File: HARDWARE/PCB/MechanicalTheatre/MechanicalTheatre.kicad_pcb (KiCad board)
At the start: 2 copper layers, 4 parts, among them U1 Teensy4.1, U2 SN74AHCT125N, U3 ESP32-DEVKITC-32D, U4 SN74HC14N

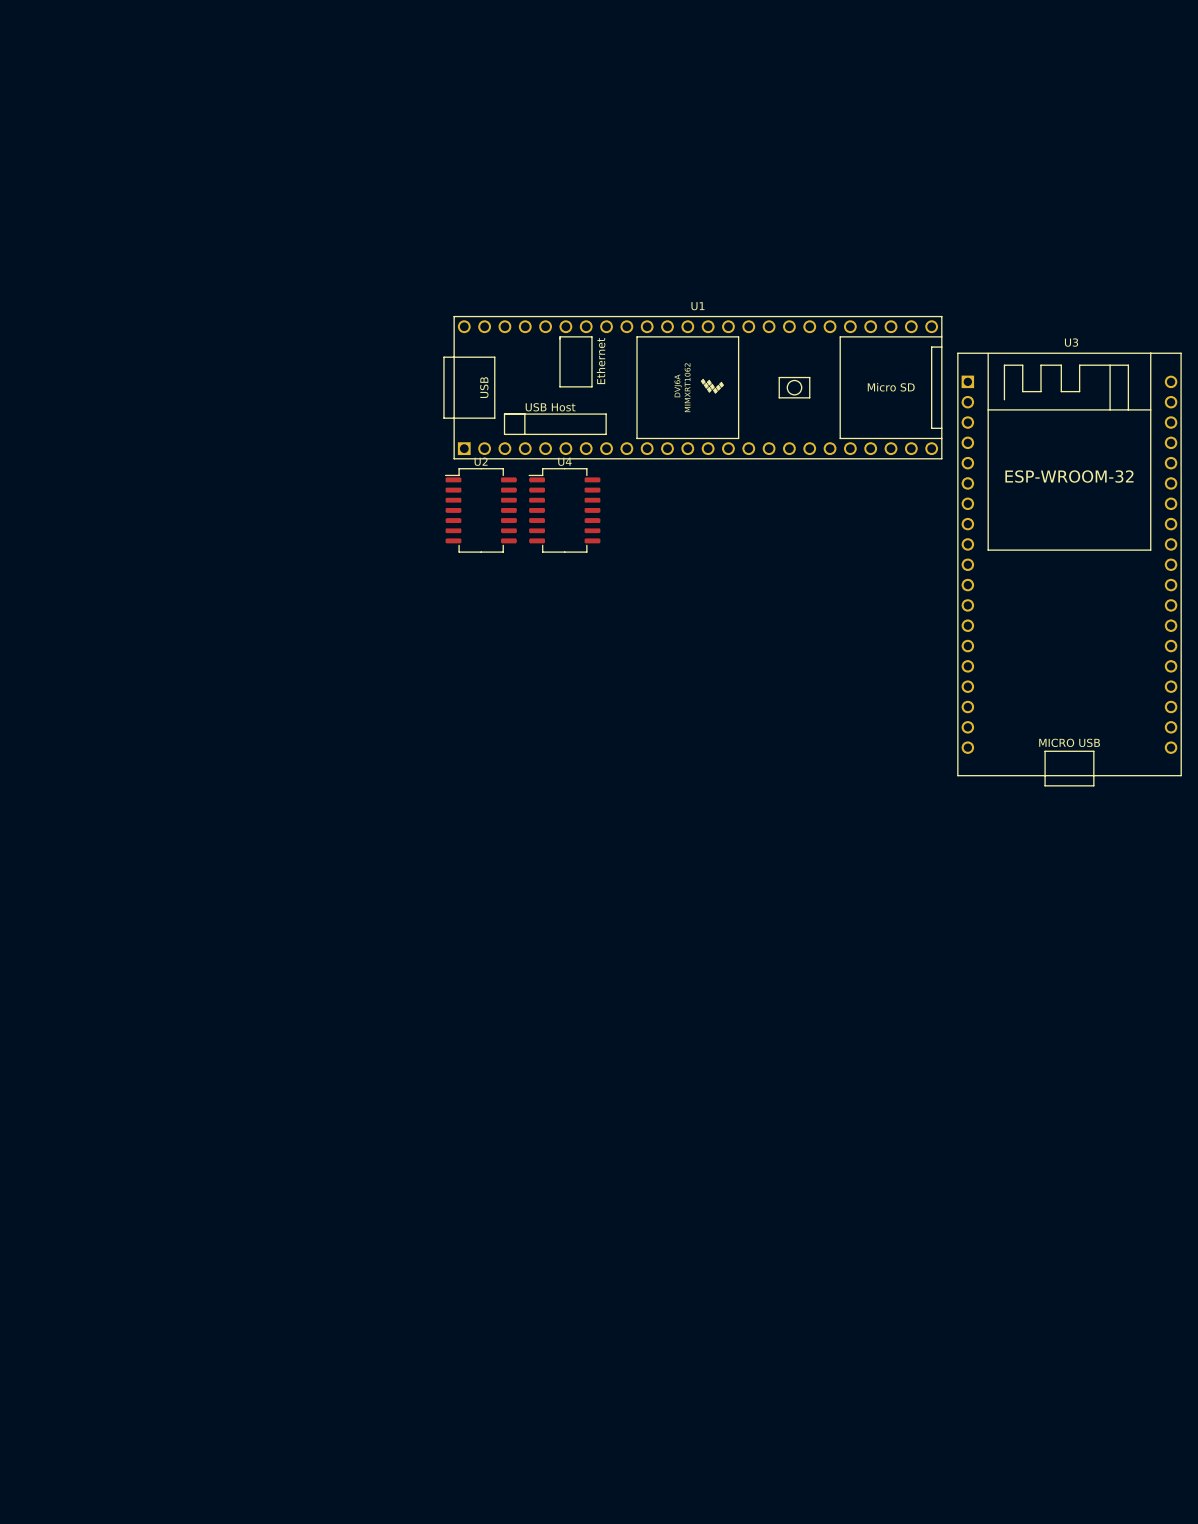
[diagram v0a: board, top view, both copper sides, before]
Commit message: main pcb v1.0
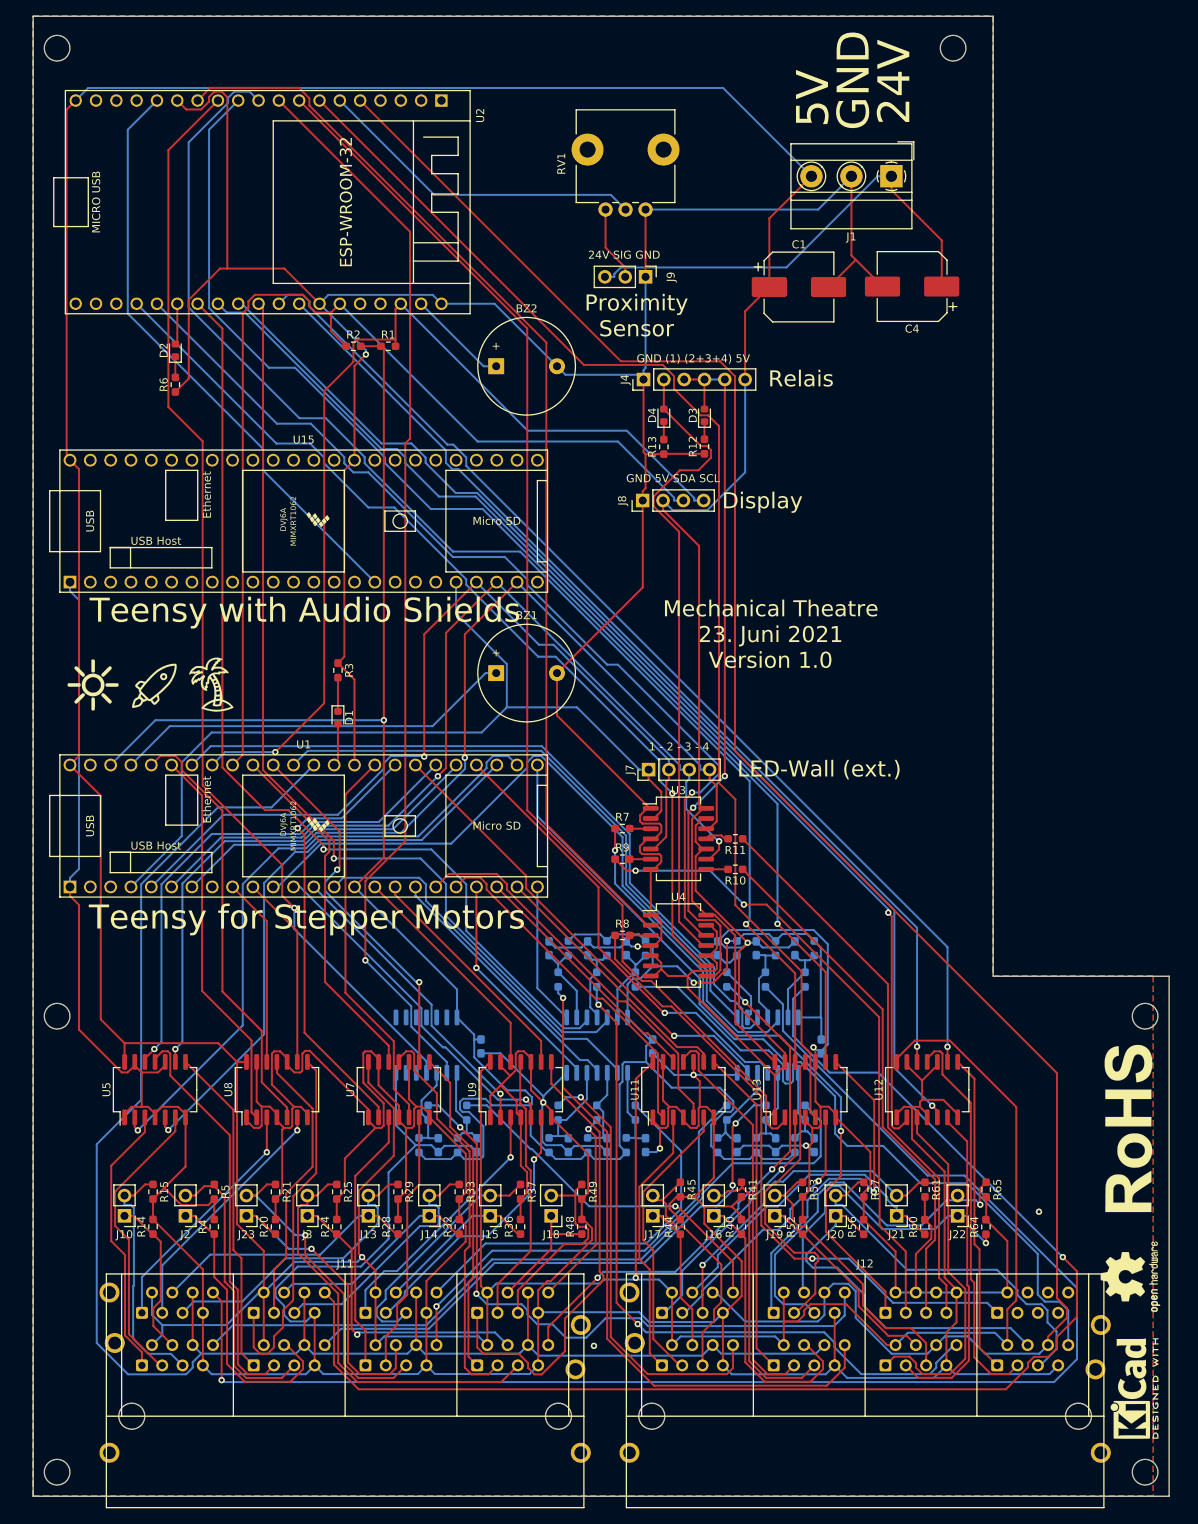
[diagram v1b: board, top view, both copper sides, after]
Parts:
- added BZ1: Buzzer, Buzzer_Beeper:Buzzer_12x9.5RM7.6, F.Cu at (87.9, 122.1)
- added BZ2: Buzzer, Buzzer_Beeper:Buzzer_12x9.5RM7.6, F.Cu at (87.9, 83.8)
- added C1: 220uF, 25V, Capacitor_SMD:CP_Elec_8x10.5, F.Cu at (125.7, 73.9)
- added C10: 0.1uF 16V, Capacitor_SMD:C_0603_1608Metric_Pad1.08x0.95mm_HandSolder, B.Cu at (107.4, 168.8)
- added C11: 0.1uF 16V, Capacitor_SMD:C_0603_1608Metric_Pad1.08x0.95mm_HandSolder, B.Cu at (106.6, 181.1)
- added C12: 0.1uF 16V, Capacitor_SMD:C_0603_1608Metric_Pad1.08x0.95mm_HandSolder, B.Cu at (94.5, 156.5)
- added C13: 0.1uF 16V, Capacitor_SMD:C_0603_1608Metric_Pad1.08x0.95mm_HandSolder, B.Cu at (96.9, 181.1)
- added C14: 0.1uF 16V, Capacitor_SMD:C_0603_1608Metric_Pad1.08x0.95mm_HandSolder, B.Cu at (101.7, 181.1)
- added C15: 0.1uF 16V, Capacitor_SMD:C_0603_1608Metric_Pad1.08x0.95mm_HandSolder, B.Cu at (99.3, 156.5)
- added C16: 0.1uF 16V, Capacitor_SMD:C_0603_1608Metric_Pad1.08x0.95mm_HandSolder, B.Cu at (104.1, 156.5)
- added C17: 0.1uF 16V, Capacitor_SMD:C_0603_1608Metric_Pad1.08x0.95mm_HandSolder, B.Cu at (86.0, 168.8)
- added C18: 0.1uF 16V, Capacitor_SMD:C_0603_1608Metric_Pad1.08x0.95mm_HandSolder, B.Cu at (85.5, 181.1)
- added C2: 0.1uF 16V, Capacitor_SMD:C_0603_1608Metric_Pad1.08x0.95mm_HandSolder, B.Cu at (122.8, 181.1)
- added C20: 0.1uF 16V, Capacitor_SMD:C_0603_1608Metric_Pad1.08x0.95mm_HandSolder, B.Cu at (80.6, 181.1)
- added C3: 0.1uF 16V, Capacitor_SMD:C_0603_1608Metric_Pad1.08x0.95mm_HandSolder, B.Cu at (118.0, 181.1)
- added C4: 220uF, 25V, Capacitor_SMD:CP_Elec_8x10.5, F.Cu at (139.9, 73.8)
- added C5: 0.1uF 16V, Capacitor_SMD:C_0603_1608Metric_Pad1.08x0.95mm_HandSolder, B.Cu at (128.5, 168.8)
- added C6: 0.1uF 16V, Capacitor_SMD:C_0603_1608Metric_Pad1.08x0.95mm_HandSolder, B.Cu at (127.6, 181.1)
- added C7: 0.1uF 16V, Capacitor_SMD:C_0603_1608Metric_Pad1.08x0.95mm_HandSolder, B.Cu at (115.6, 156.5)
- added C8: 0.1uF 16V, Capacitor_SMD:C_0603_1608Metric_Pad1.08x0.95mm_HandSolder, B.Cu at (120.4, 156.5)
- added C9: 0.1uF 16V, Capacitor_SMD:C_0603_1608Metric_Pad1.08x0.95mm_HandSolder, B.Cu at (125.2, 156.5)
- added D1: LED, LED_SMD:LED_0603_1608Metric, F.Cu at (68.1, 127.7)
- added D2: LED, LED_SMD:LED_0603_1608Metric, F.Cu at (47.8, 81.8)
- added D3: LED, LED_SMD:LED_0603_1608Metric, F.Cu at (113.9, 89.9)
- added D4: LED, LED_SMD:LED_0603_1608Metric, F.Cu at (108.8, 89.9)
- added G***: LOGO, Clockdiv-Logos:sunrocketpalmtree_21.7mm, F.Cu at (44.7, 123.9)
- added J1: Power In 5V/24V, TerminalBlock_MetzConnect:TerminalBlock_MetzConnect_Type011_RT05503HBWC_1x03_P5.00mm_Horizontal, F.Cu at (137.3, 60.0)
- added J10: Conn_01x02_General Purpose 01, Connector_PinHeader_2.54mm:PinHeader_1x02_P2.54mm_Vertical, F.Cu at (41.4, 190.0)
- added J11: RJ45 8x Socket, Clockdiv-KiCad:RJ45_Conrad_8x, F.Cu at (69.0, 215.0)
- added J12: RJ45 8x Socket, Clockdiv-KiCad:RJ45_Conrad_8x, F.Cu at (134.0, 215.0)
- added J13: Conn_01x02_General Purpose 05, Connector_PinHeader_2.54mm:PinHeader_1x02_P2.54mm_Vertical, F.Cu at (71.9, 190.0)
- added J14: Conn_01x02_General Purpose 06, Connector_PinHeader_2.54mm:PinHeader_1x02_P2.54mm_Vertical, F.Cu at (79.5, 190.0)
- added J15: Conn_01x02_General Purpose 07, Connector_PinHeader_2.54mm:PinHeader_1x02_P2.54mm_Vertical, F.Cu at (87.1, 190.0)
- added J16: Conn_01x02_General Purpose 10, Connector_PinHeader_2.54mm:PinHeader_1x02_P2.54mm_Vertical, F.Cu at (115.1, 190.0)
- added J17: Conn_01x02_General Purpose 09, Connector_PinHeader_2.54mm:PinHeader_1x02_P2.54mm_Vertical, F.Cu at (107.5, 190.0)
- added J18: Conn_01x02_General Purpose 08, Connector_PinHeader_2.54mm:PinHeader_1x02_P2.54mm_Vertical, F.Cu at (94.8, 190.0)
- added J19: Conn_01x02_General Purpose 11, Connector_PinHeader_2.54mm:PinHeader_1x02_P2.54mm_Vertical, F.Cu at (122.7, 190.0)
- added J2: Conn_01x02_General Purpose 02, Connector_PinHeader_2.54mm:PinHeader_1x02_P2.54mm_Vertical, F.Cu at (49.0, 190.0)
- added J20: Conn_01x02_General Purpose 12, Connector_PinHeader_2.54mm:PinHeader_1x02_P2.54mm_Vertical, F.Cu at (130.3, 190.0)
- added J21: Conn_01x02_General Purpose 13, Connector_PinHeader_2.54mm:PinHeader_1x02_P2.54mm_Vertical, F.Cu at (137.9, 190.0)
- added J22: Conn_01x02_General Purpose 14, Connector_PinHeader_2.54mm:PinHeader_1x02_P2.54mm_Vertical, F.Cu at (145.6, 190.0)
- added J23: Conn_01x02_General Purpose 03, Connector_PinHeader_2.54mm:PinHeader_1x02_P2.54mm_Vertical, F.Cu at (56.7, 190.0)
- added J3: Conn_01x02_General Purpose 04, Connector_PinHeader_2.54mm:PinHeader_1x02_P2.54mm_Vertical, F.Cu at (64.3, 190.0)
- added J4: Conn_01x06_Relais, Connector_PinHeader_2.54mm:PinHeader_1x06_P2.54mm_Vertical, F.Cu at (106.3, 85.4)
- added J7: Conn_01x04_WS2812B, Connector_PinHeader_2.54mm:PinHeader_1x04_P2.54mm_Vertical, F.Cu at (106.9, 134.2)
- added J8: Conn_01x04_I2C_Display_20x4, Connector_PinHeader_2.54mm:PinHeader_1x04_P2.54mm_Vertical, F.Cu at (106.2, 100.5)
- added J9: Conn_01x03_ProximitySensor, Connector_PinHeader_2.54mm:PinHeader_1x03_P2.54mm_Vertical, F.Cu at (106.6, 72.6)
- added R1: 4.7k, Resistor_SMD:R_0603_1608Metric_Pad0.98x0.95mm_HandSolder, F.Cu at (74.4, 81.3)
- added R10: 100, Resistor_SMD:R_0603_1608Metric_Pad0.98x0.95mm_HandSolder, F.Cu at (117.8, 146.6)
- added R11: 100, Resistor_SMD:R_0603_1608Metric_Pad0.98x0.95mm_HandSolder, F.Cu at (117.8, 142.8)
- added R12: 120, Resistor_SMD:R_0603_1608Metric_Pad0.98x0.95mm_HandSolder, F.Cu at (113.9, 93.8)
- added R13: 120, Resistor_SMD:R_0603_1608Metric_Pad0.98x0.95mm_HandSolder, F.Cu at (108.8, 93.8)
- added R14: 10k, Resistor_SMD:R_0603_1608Metric_Pad0.98x0.95mm_HandSolder, F.Cu at (45.0, 191.3)
- added R15: 10k, Resistor_SMD:R_0603_1608Metric_Pad0.98x0.95mm_HandSolder, F.Cu at (45.0, 186.9)
- added R16: 10k, Resistor_SMD:R_0603_1608Metric_Pad0.98x0.95mm_HandSolder, B.Cu at (125.2, 181.1)
- added R17: 1k, Resistor_SMD:R_0603_1608Metric_Pad0.98x0.95mm_HandSolder, B.Cu at (126.5, 177.1)
- added R18: 10k, Resistor_SMD:R_0603_1608Metric_Pad0.98x0.95mm_HandSolder, B.Cu at (120.4, 181.1)
- added R19: 1k, Resistor_SMD:R_0603_1608Metric_Pad0.98x0.95mm_HandSolder, B.Cu at (121.6, 177.1)
- added R2: 4.7k, Resistor_SMD:R_0603_1608Metric_Pad0.98x0.95mm_HandSolder, F.Cu at (70.0, 81.3)
- added R20: 10k, Resistor_SMD:R_0603_1608Metric_Pad0.98x0.95mm_HandSolder, F.Cu at (60.3, 191.3)
- added R21: 10k, Resistor_SMD:R_0603_1608Metric_Pad0.98x0.95mm_HandSolder, F.Cu at (60.3, 186.9)
- added R22: 10k, Resistor_SMD:R_0603_1608Metric_Pad0.98x0.95mm_HandSolder, B.Cu at (115.6, 181.1)
- added R23: 1k, Resistor_SMD:R_0603_1608Metric_Pad0.98x0.95mm_HandSolder, B.Cu at (116.7, 177.1)
- added R24: 10k, Resistor_SMD:R_0603_1608Metric_Pad0.98x0.95mm_HandSolder, F.Cu at (68.0, 191.3)
- added R25: 10k, Resistor_SMD:R_0603_1608Metric_Pad0.98x0.95mm_HandSolder, F.Cu at (68.0, 186.9)
- added R26: 10k, Resistor_SMD:R_0603_1608Metric_Pad0.98x0.95mm_HandSolder, B.Cu at (118.0, 156.5)
- added R27: 1k, Resistor_SMD:R_0603_1608Metric_Pad0.98x0.95mm_HandSolder, B.Cu at (116.7, 160.4)
- added R28: 10k, Resistor_SMD:R_0603_1608Metric_Pad0.98x0.95mm_HandSolder, F.Cu at (75.6, 191.3)
- added R29: 10k, Resistor_SMD:R_0603_1608Metric_Pad0.98x0.95mm_HandSolder, F.Cu at (75.6, 186.9)
- added R3: 220, Resistor_SMD:R_0603_1608Metric_Pad0.98x0.95mm_HandSolder, F.Cu at (68.1, 121.8)
- added R30: 10k, Resistor_SMD:R_0603_1608Metric_Pad0.98x0.95mm_HandSolder, B.Cu at (122.8, 156.5)
- added R31: 1k, Resistor_SMD:R_0603_1608Metric_Pad0.98x0.95mm_HandSolder, B.Cu at (121.5, 160.4)
- added R32: 10k, Resistor_SMD:R_0603_1608Metric_Pad0.98x0.95mm_HandSolder, F.Cu at (83.3, 191.3)
- added R33: 10k, Resistor_SMD:R_0603_1608Metric_Pad0.98x0.95mm_HandSolder, F.Cu at (83.3, 186.9)
- added R34: 10k, Resistor_SMD:R_0603_1608Metric_Pad0.98x0.95mm_HandSolder, B.Cu at (127.6, 156.5)
- added R35: 1k, Resistor_SMD:R_0603_1608Metric_Pad0.98x0.95mm_HandSolder, B.Cu at (126.5, 160.4)
- added R36: 10k, Resistor_SMD:R_0603_1608Metric_Pad0.98x0.95mm_HandSolder, F.Cu at (90.9, 191.3)
- added R37: 10k, Resistor_SMD:R_0603_1608Metric_Pad0.98x0.95mm_HandSolder, F.Cu at (90.9, 186.9)
- added R38: 10k, Resistor_SMD:R_0603_1608Metric_Pad0.98x0.95mm_HandSolder, B.Cu at (104.1, 181.1)
- added R39: 1k, Resistor_SMD:R_0603_1608Metric_Pad0.98x0.95mm_HandSolder, B.Cu at (105.3, 177.1)
- added R4: 10k, Resistor_SMD:R_0603_1608Metric_Pad0.98x0.95mm_HandSolder, F.Cu at (52.6, 191.3)
- added R40: 10k, Resistor_SMD:R_0603_1608Metric_Pad0.98x0.95mm_HandSolder, F.Cu at (118.5, 191.3)
- added R41: 10k, Resistor_SMD:R_0603_1608Metric_Pad0.98x0.95mm_HandSolder, F.Cu at (118.5, 186.7)
- added R42: 10k, Resistor_SMD:R_0603_1608Metric_Pad0.98x0.95mm_HandSolder, B.Cu at (96.9, 156.5)
- added R43: 1k, Resistor_SMD:R_0603_1608Metric_Pad0.98x0.95mm_HandSolder, B.Cu at (95.6, 160.4)
- added R44: 10k, Resistor_SMD:R_0603_1608Metric_Pad0.98x0.95mm_HandSolder, F.Cu at (110.9, 191.3)
- added R45: 10k, Resistor_SMD:R_0603_1608Metric_Pad0.98x0.95mm_HandSolder, F.Cu at (110.9, 186.7)
- added R46: 10k, Resistor_SMD:R_0603_1608Metric_Pad0.98x0.95mm_HandSolder, B.Cu at (94.5, 181.1)
- added R47: 1k, Resistor_SMD:R_0603_1608Metric_Pad0.98x0.95mm_HandSolder, B.Cu at (95.6, 177.1)
- added R48: 10k, Resistor_SMD:R_0603_1608Metric_Pad0.98x0.95mm_HandSolder, F.Cu at (98.6, 191.3)
- added R49: 10k, Resistor_SMD:R_0603_1608Metric_Pad0.98x0.95mm_HandSolder, F.Cu at (98.6, 186.9)
- added R5: 10k, Resistor_SMD:R_0603_1608Metric_Pad0.98x0.95mm_HandSolder, F.Cu at (52.6, 186.9)
- added R50: 10k, Resistor_SMD:R_0603_1608Metric_Pad0.98x0.95mm_HandSolder, B.Cu at (99.3, 181.1)
- added R51: 1k, Resistor_SMD:R_0603_1608Metric_Pad0.98x0.95mm_HandSolder, B.Cu at (100.5, 177.1)
- added R52: 10k, Resistor_SMD:R_0603_1608Metric_Pad0.98x0.95mm_HandSolder, F.Cu at (126.2, 191.3)
- added R53: 10k, Resistor_SMD:R_0603_1608Metric_Pad0.98x0.95mm_HandSolder, F.Cu at (126.2, 186.7)
- added R54: 10k, Resistor_SMD:R_0603_1608Metric_Pad0.98x0.95mm_HandSolder, B.Cu at (101.7, 156.5)
- added R55: 1k, Resistor_SMD:R_0603_1608Metric_Pad0.98x0.95mm_HandSolder, B.Cu at (100.5, 160.4)
- added R56: 10k, Resistor_SMD:R_0603_1608Metric_Pad0.98x0.95mm_HandSolder, F.Cu at (133.8, 191.3)
- added R57: 10k, Resistor_SMD:R_0603_1608Metric_Pad0.98x0.95mm_HandSolder, F.Cu at (133.8, 186.7)
- added R58: 10k, Resistor_SMD:R_0603_1608Metric_Pad0.98x0.95mm_HandSolder, B.Cu at (106.6, 156.5)
- added R59: 1k, Resistor_SMD:R_0603_1608Metric_Pad0.98x0.95mm_HandSolder, B.Cu at (105.3, 160.4)
- added R6: 120, Resistor_SMD:R_0603_1608Metric_Pad0.98x0.95mm_HandSolder, F.Cu at (47.8, 86.1)
- added R60: 10k, Resistor_SMD:R_0603_1608Metric_Pad0.98x0.95mm_HandSolder, F.Cu at (141.5, 191.3)
- added R61: 10k, Resistor_SMD:R_0603_1608Metric_Pad0.98x0.95mm_HandSolder, F.Cu at (141.5, 186.7)
- added R62: 10k, Resistor_SMD:R_0603_1608Metric_Pad0.98x0.95mm_HandSolder, B.Cu at (83.1, 181.1)
- added R63: 1k, Resistor_SMD:R_0603_1608Metric_Pad0.98x0.95mm_HandSolder, B.Cu at (84.2, 177.1)
- added R64: 10k, Resistor_SMD:R_0603_1608Metric_Pad0.98x0.95mm_HandSolder, F.Cu at (149.1, 191.3)
- added R65: 10k, Resistor_SMD:R_0603_1608Metric_Pad0.98x0.95mm_HandSolder, F.Cu at (149.1, 186.7)
- added R66: 10k, Resistor_SMD:R_0603_1608Metric_Pad0.98x0.95mm_HandSolder, B.Cu at (78.2, 181.1)
- added R67: 1k, Resistor_SMD:R_0603_1608Metric_Pad0.98x0.95mm_HandSolder, B.Cu at (79.4, 177.1)
- added R7: 100, Resistor_SMD:R_0603_1608Metric_Pad0.98x0.95mm_HandSolder, F.Cu at (103.7, 141.5)
- added R8: 100, Resistor_SMD:R_0603_1608Metric_Pad0.98x0.95mm_HandSolder, F.Cu at (103.7, 154.9)
- added R9: 100, Resistor_SMD:R_0603_1608Metric_Pad0.98x0.95mm_HandSolder, F.Cu at (103.7, 145.4)
- added REF**: OSHW-Logo2_9.8x8mm_SilkScreen, Symbol:OSHW-Logo2_9.8x8mm_SilkScreen, F.Cu at (167.2, 197.6)
- added REF**: KiCad-Logo2_5mm_SilkScreen, Symbol:KiCad-Logo2_5mm_SilkScreen, F.Cu at (167.7, 211.5)
- added REF**: RoHS-Logo_6mm_SilkScreen, Symbol:RoHS-Logo_6mm_SilkScreen, F.Cu at (166.9, 179.0)
- added RV1: R_POT, Potentiometer_THT:Potentiometer_Alps_RK09L_Single_Vertical, F.Cu at (106.6, 64.2)
- added U10: SN74HC14S, Package_SO:SO-14_5.3x10.2mm_P1.27mm, B.Cu at (100.5, 168.6)
- added U11: SN74AHCT125N, Package_SO:SO-14_5.3x10.2mm_P1.27mm, F.Cu at (111.3, 174.2)
- added U12: SN74AHCT125N, Package_SO:SO-14_5.3x10.2mm_P1.27mm, F.Cu at (141.8, 174.2)
- added U13: SN74AHCT125N, Package_SO:SO-14_5.3x10.2mm_P1.27mm, F.Cu at (126.5, 174.2)
- added U14: SN74HC14S, Package_SO:SO-14_5.3x10.2mm_P1.27mm, B.Cu at (79.2, 168.6)
- added U15: Teensy4.1_OuterPins, teensy:Teensy41_OuterPinsOnly, F.Cu at (63.8, 103.1)
- added U5: SN74AHCT125N, Package_SO:SO-14_5.3x10.2mm_P1.27mm, F.Cu at (45.2, 174.2)
- added U6: SN74HC14S, Package_SO:SO-14_5.3x10.2mm_P1.27mm, B.Cu at (121.8, 168.6)
- added U7: SN74AHCT125N, Package_SO:SO-14_5.3x10.2mm_P1.27mm, F.Cu at (75.7, 174.2)
- added U8: SN74AHCT125N, Package_SO:SO-14_5.3x10.2mm_P1.27mm, F.Cu at (60.5, 174.2)
- added U9: SN74AHCT125N, Package_SO:SO-14_5.3x10.2mm_P1.27mm, F.Cu at (91.0, 174.2)
- U1: value Teensy4.1 -> Teensy4.1_OuterPins
- U2: value SN74AHCT125N -> ESP32-DEVKITC-32D; footprint Package_SO:SO-14_5.3x10.2mm_P1.27mm -> ESP32-DEVKITC-32D:MODULE_ESP32-DEVKITC-32D
- U3: value ESP32-DEVKITC-32D -> SN74AHCT125N; footprint ESP32-DEVKITC-32D:MODULE_ESP32-DEVKITC-32D -> Package_SO:SO-14_5.3x10.2mm_P1.27mm
- U4: value SN74HC14N -> SN74AHCT125N
- moved U1 73.7 mm to (63.8, 141.2)
- moved U3 61.5 mm to (110.7, 142.8)
- moved U4 56.2 mm to (110.7, 156.2)
- moved U2 45.8 mm to (61.3, 63.2), turned to 270 degrees
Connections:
- U1 pad 1: Net-(U1-Pad1) -> GND
- U1 pad 10: Net-(U1-Pad10) -> /STEPPER_6_DIR
- U1 pad 11: Net-(U1-Pad11) -> /STEPPER_6_END
- U1 pad 12: Net-(U1-Pad12) -> /STEPPER_7_STEP
- U1 pad 13: Net-(U1-Pad13) -> /STEPPER_7_DIR
- U1 pad 14: Net-(U1-Pad14) -> /STEPPER_7_END
- U1 pad 15: Net-(U1-Pad15) -> +3V3
- U1 pad 16: Net-(U1-Pad16) -> /STEPPER_8_STEP
- U1 pad 17: Net-(U1-Pad17) -> /STEPPER_8_DIR
- U1 pad 18: Net-(U1-Pad18) -> /STEPPER_8_END
- U1 pad 19: Net-(U1-Pad19) -> /STEPPER_9_STEP
- U1 pad 20: Net-(U1-Pad20) -> /STEPPER_9_DIR
- U1 pad 21: Net-(U1-Pad21) -> /STEPPER_9_END
- U1 pad 22: Net-(U1-Pad22) -> /STEPPER_10_STEP
- U1 pad 23: Net-(U1-Pad23) -> /STEPPER_10_DIR
- U1 pad 24: Net-(U1-Pad24) -> /STEPPER_10_END
- U1 pad 25: Net-(U1-Pad25) -> /STEPPER_1_END
- U1 pad 26: Net-(U1-Pad26) -> /STEPPER_1_DIR
- U1 pad 27: Net-(U1-Pad27) -> /STEPPER_1_STEP
- U1 pad 28: Net-(U1-Pad28) -> /STEPPER_2_END
- U1 pad 29: Net-(U1-Pad29) -> /STEPPER_2_DIR
- U1 pad 30: Net-(U1-Pad30) -> /STEPPER_2_STEP
- U1 pad 31: Net-(U1-Pad31) -> /STEPPER_3_END
- U1 pad 32: Net-(U1-Pad32) -> /STEPPER_3_DIR
- U1 pad 33: Net-(U1-Pad33) -> /STEPPER_3_STEP
- U1 pad 34: Net-(U1-Pad34) -> GND
- U1 pad 36: Net-(U1-Pad36) -> /GENERAL_END_SWITCH_TEENSY
- U1 pad 37: Net-(U1-Pad37) -> /STEPPER_4_END
- U1 pad 38: Net-(U1-Pad38) -> /STEPPER_4_DIR
- U1 pad 39: Net-(U1-Pad39) -> /STEPPER_4_STEP
- U1 pad 4: Net-(U1-Pad4) -> /WS2812B_Line_1
- U1 pad 40: Net-(U1-Pad40) -> /I2C_SDA
- U1 pad 41: Net-(U1-Pad41) -> /I2C_SCL
- U1 pad 42: Net-(U1-Pad42) -> /STEPPER_5_END
- U1 pad 43: Net-(U1-Pad43) -> /STEPPER_5_DIR
- U1 pad 44: Net-(U1-Pad44) -> /STEPPER_5_STEP
- U1 pad 46: Net-(U1-Pad46) -> +3V3
- U1 pad 48: Net-(U1-Pad48) -> +5V
- U1 pad 5: Net-(U1-Pad5) -> /WS2812B_Line_2
- U1 pad 6: Net-(U1-Pad6) -> /WS2812B_Line_3
- U1 pad 7: Net-(U1-Pad7) -> /WS2812B_Line_4
- U1 pad 9: Net-(U1-Pad9) -> /STEPPER_6_STEP
- U2 pad 10: Net-(U2-Pad10) -> /STEPPER_14_STEP
- U2 pad 11: Net-(U2-Pad11) -> /STEPPER_14_DIR
- U2 pad 12: Net-(U2-Pad12) -> /STEPPER_14_END
- U2 pad 13: Net-(U2-Pad13) -> /WS2812B_LED_LIGHTING
- U2 pad 14: Net-(U2-Pad14) -> GND
- U2 pad 5: Net-(U2-Pad5) -> /GENERAL_END_SWITCH_ESP32
- U2 pad 6: Net-(U2-Pad6) -> /PROX_SENSOR
- U2 pad 7: Net-(U2-Pad7) -> /STEPPER_13_STEP
- U2 pad 8: Net-(U2-Pad8) -> /STEPPER_13_DIR
- U2 pad 9: Net-(U2-Pad9) -> /STEPPER_13_END
- U3 pad 1: Net-(U3-Pad1) -> GND
- U3 pad 10: Net-(U3-Pad10) -> GND
- U3 pad 12: Net-(U3-Pad12) -> /WS2812B_Line_4
- U3 pad 13: Net-(U3-Pad13) -> GND
- U3 pad 14: Net-(U3-Pad14) -> +5V
- U3 pad 2: Net-(U3-Pad2) -> /WS2812B_Line_1
- U3 pad 4: Net-(U3-Pad4) -> GND
- U3 pad 5: Net-(U3-Pad5) -> /WS2812B_Line_2
- U3 pad 7: Net-(U3-Pad7) -> GND
- U3 pad 9: Net-(U3-Pad9) -> /WS2812B_Line_3
- U4 pad 1: Net-(U4-Pad1) -> GND
- U4 pad 10: Net-(U4-Pad10) -> GND
- U4 pad 12: Net-(U4-Pad12) -> /RELAIS_E-MAGNET
- U4 pad 13: Net-(U4-Pad13) -> GND
- U4 pad 14: Net-(U4-Pad14) -> +5V
- U4 pad 2: Net-(U4-Pad2) -> /WS2812B_LED_LIGHTING
- U4 pad 4: Net-(U4-Pad4) -> GND
- U4 pad 5: Net-(U4-Pad5) -> GND
- U4 pad 7: Net-(U4-Pad7) -> GND
- U4 pad 9: Net-(U4-Pad9) -> /RELAIS_24V+5V
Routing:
- net GND: track 0.00 -> 1309.3 mm, vias 0 -> 10
- net +5V: track 0.00 -> 695.6 mm, vias 0 -> 2
- net +3V3: track 0.00 -> 311.1 mm, vias 0 -> 3
- net /GENERAL_END_SWITCH_ESP32: track 0.00 -> 255.2 mm
- net /GENERAL_END_SWITCH_TEENSY: track 0.00 -> 213.5 mm
- net Net-(J11-Pad58): track 0.00 -> 185.0 mm, vias 0 -> 1
- net Net-(J11-Pad68): track 0.00 -> 168.7 mm, vias 0 -> 1
- net /STEPPER_14_STEP: track 0.00 -> 165.8 mm, vias 0 -> 1
- net /STEPPER_14_DIR: track 0.00 -> 159.3 mm, vias 0 -> 1
- net /STEPPER_13_STEP: track 0.00 -> 159.1 mm
- net /STEPPER_13_DIR: track 0.00 -> 156.1 mm
- net /STEPPER_11_DIR: track 0.00 -> 145.7 mm, vias 0 -> 1
- net /STEPPER_11_STEP: track 0.00 -> 141.9 mm, vias 0 -> 1
- net /STEPPER_14_END: track 0.00 -> 137.5 mm, vias 0 -> 1
- net /WS2812B_LED_LIGHTING: track 0.00 -> 136.5 mm
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- added copper zone on B.Cu, net GND
- added copper zone on F.Cu, net GND
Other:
- board outline added: 142 x 185 mm
- board text added: "1 - 2 - 3 - 4"
- board text added: "24V"
- board text added: "24V SIG GND"
- board text added: "5V"
- board text added: "Display"
- board text added: "GND"
- board text added: "GND (1) (2+3+4) 5V"
- board text added: "GND 5V SDA SCL"
- board text added: "LED-Wall (ext.)"
- board text added: "Mechanical Theatre 23. Juni 2021 Version 1.0"
- board text added: "Proximity Sensor"
- board text added: "Relais"
- board text added: "Teensy for Stepper Motors"
- board text added: "Teensy with Audio Shields"
